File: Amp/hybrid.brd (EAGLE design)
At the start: 174 x 168.9 mm, 123 parts, among them IC1 TL071P, IC2 TL071P, IC3 LM317MABT-OUT, IC4 LM317MABT-OUT, J1 RCJ-21XXMILL, J2 NRJ3HF-1, J3 703W-00/54, Q1 BC560KINKED, Q10 BC560KINKED, Q11 BC560KINKED, Q12 BC560KINKED, Q13 BC556KINKED, Q14 BC550KINKED, Q15 BC550KINKED, Q16 BC560KINKED, Q17 BD140, Q18 BD139, Q19 KSP43, Q2 BC560KINKED, Q3 BC560KINKED, Q4 BC556KINKED, Q5 BC550KINKED, Q6 BC550KINKED, Q7 BC560KINKED, Q8 BD140, Q9 BD139, T1 TR-LP30-1600

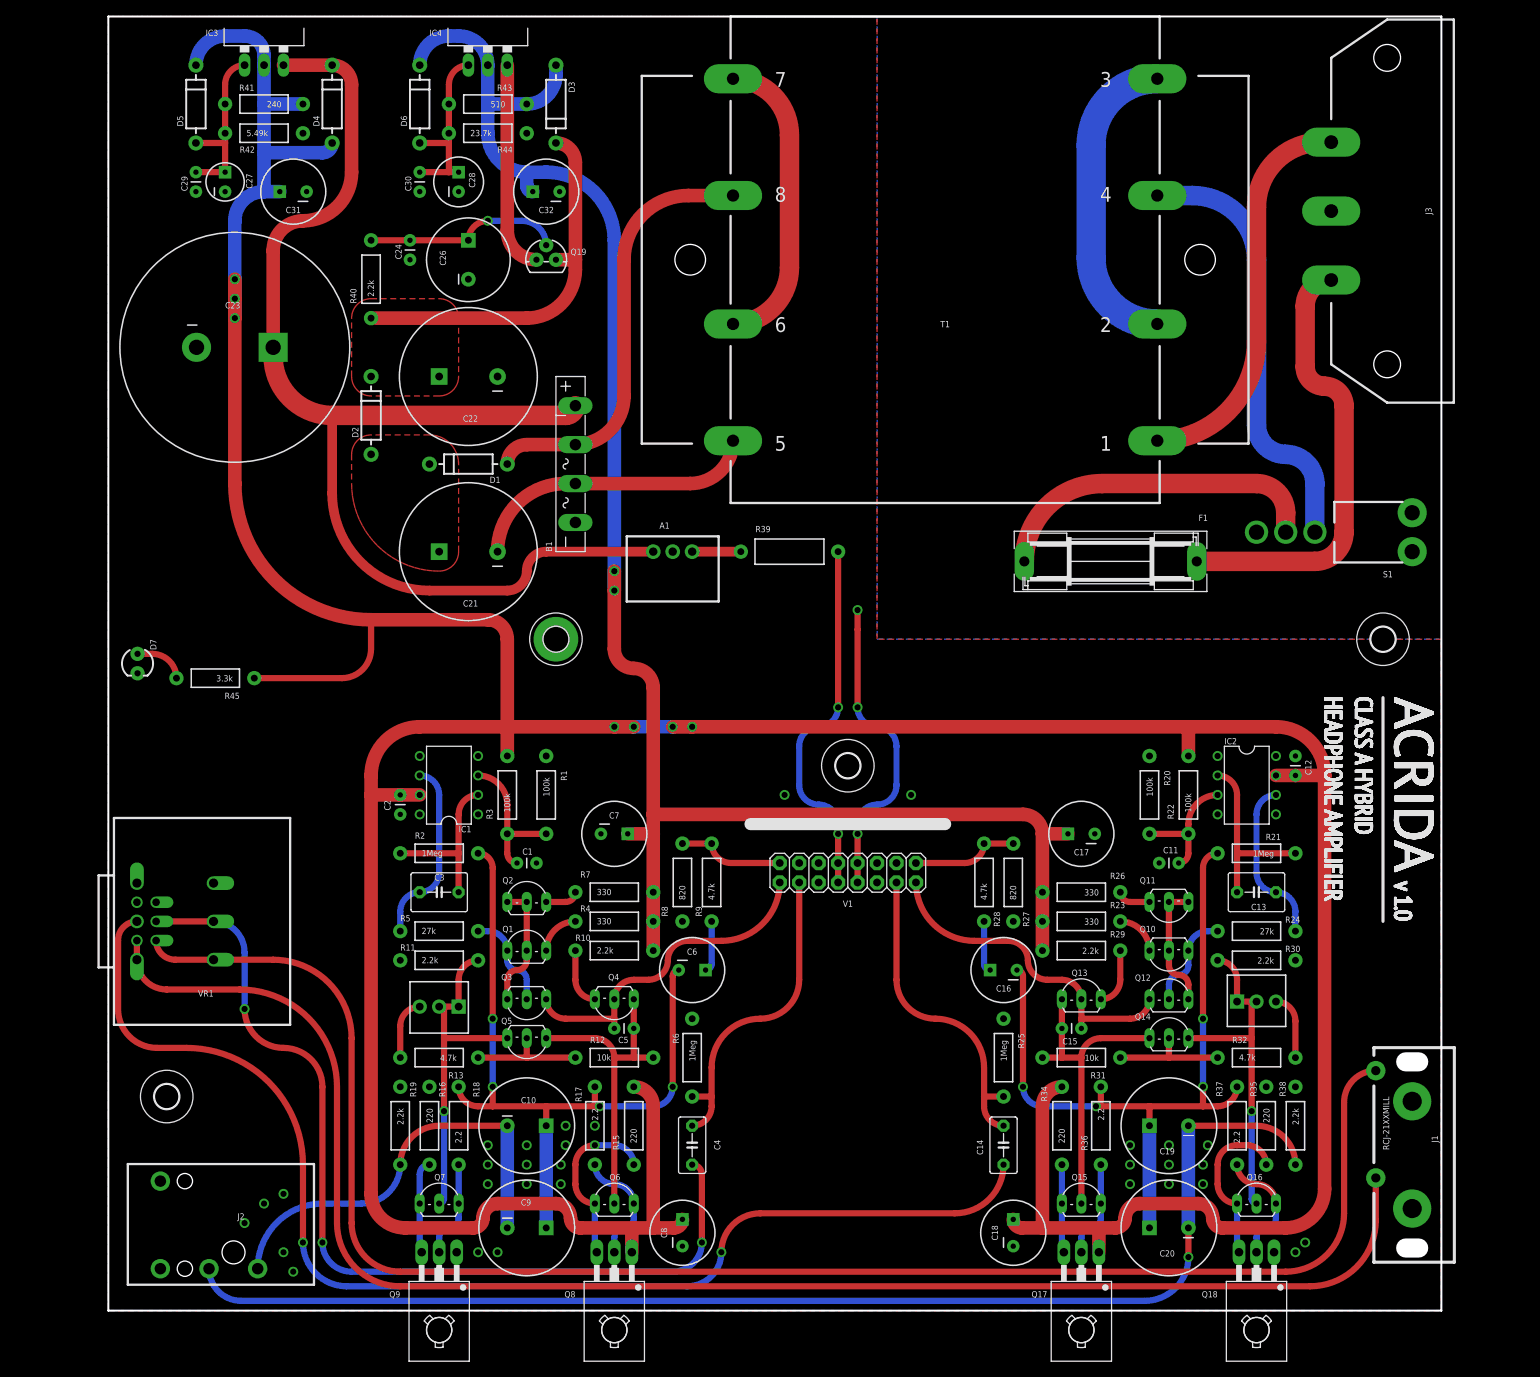
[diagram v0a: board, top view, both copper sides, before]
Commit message: Small changes
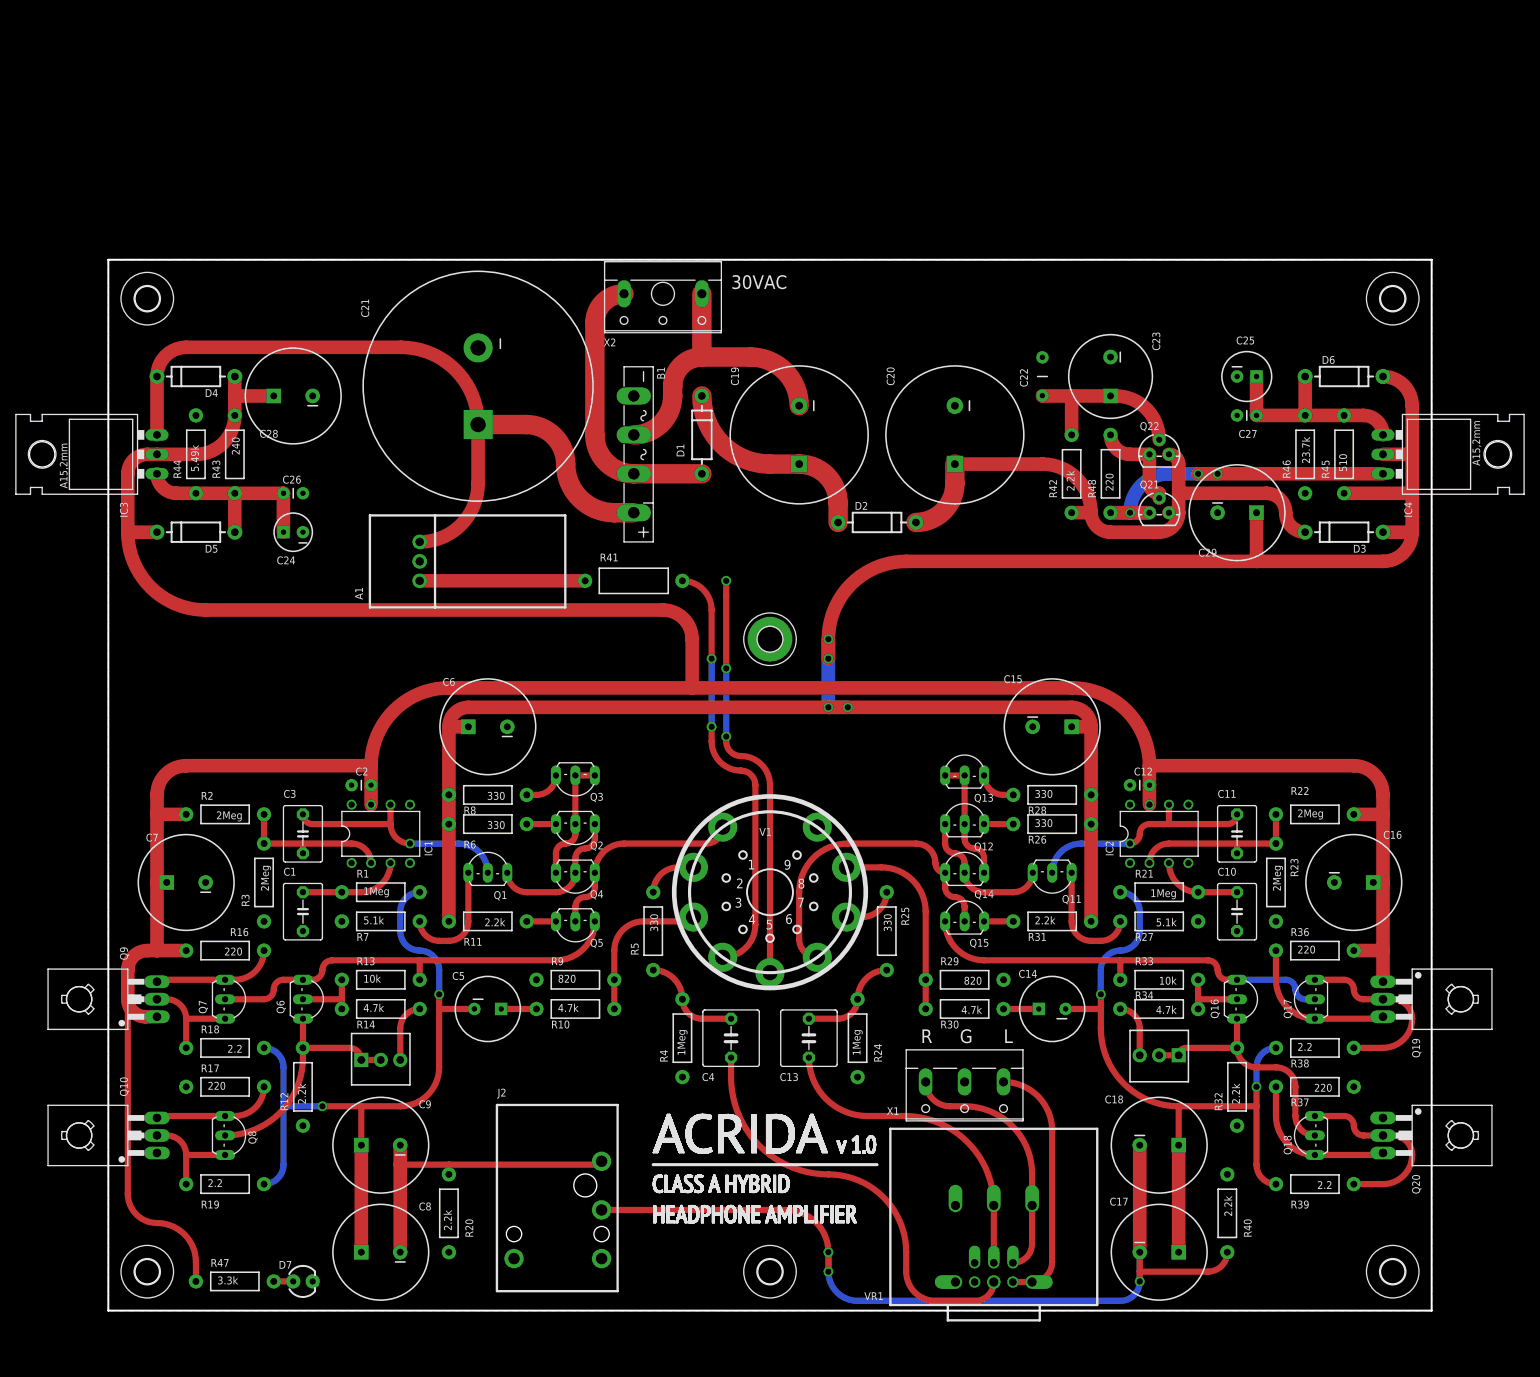
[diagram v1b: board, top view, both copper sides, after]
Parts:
- removed C30: 1uF, SparkFun-Capacitors:CAP-PTH-SMALL
- removed C31, C32: 47uF, my-cap:CPOL-RADIAL-8/3.5
- removed F1: (no value), fuse:SH22,5
- removed J1: RCJ-21XXMILL, my:RCJ-21-MILL
- removed J3: 703W-00/54, my-conn:703W-00/54
- removed S1: SW-M2012SA2W40, my-sw:SW-M2012S2A2G40
- removed T1: TR-LP30-1600, my-transformers:TR-LP30-1600
- removed U$1: ACRIDA-LOGO, my-logo:ACRIDA-LOGO
- removed U$2: (no value), my-logo:DANGER-LOGO
- added C25: 10uF, my-cap:CPOL-RADIAL-6.5/2.5
- added H1: MOUNT-PAD-ROUND3.2, holes:3,2-PAD
- added H6: MOUNT-HOLE3.2, holes:3,2
- added LOGO1: ACRIDA-LOGO, my-logo:ACRIDA-LOGO
- added Q20: BD139, transistor-npn:TO126
- added Q21, Q22: KSP43, my-tran:TO-92
- added R46: 23.7k, SparkFun-Resistors:AXIAL-0.4
- added R47: 3.3k, SparkFun-Resistors:AXIAL-0.4
- added R48: 220, SparkFun-Resistors:AXIAL-0.4
- added X1: (no value), con-wago-508:W237-3E
- added X2: (no value), con-wago-508:W237-2N
- C1, C11: value 0.1uF -> 1uF; device SparkFun-Capacitors:CAP-PTH-SMALL -> capacitor-wima:C5B5
- C10: value 470uF -> 1uF; device my-cap:CPOL-RADIAL-12.5/5 -> capacitor-wima:C5B5
- C12, C2: value 0.1uF -> 1uF
- C13: value 1uF -> 0.33u; device capacitor-wima:C5B5 -> capacitor-wima:C5B7.2
- C14: value 0.33u -> 100uF; device capacitor-wima:C5B3.5 -> my-cap:CPOL-RADIAL-8/3.5
- C15: value 10p -> 100uF; device SparkFun-Capacitors:CAP-PTH-SMALL -> my-cap:CPOL-RADIAL-12.5/5
- C16, C6: device my-cap:CPOL-RADIAL-8/3.5 -> my-cap:CPOL-RADIAL-12.5/5
- C17, C18, C8: value 47uF -> 470uF; device my-cap:CPOL-RADIAL-8/3.5 -> my-cap:CPOL-RADIAL-12.5/5
- C19, C20: device my-cap:CPOL-RADIAL-12.5/5 -> my-cap:CPOL-RADIAL-18/7.5
- C21: value 470uF -> 4700uF; device my-cap:CPOL-RADIAL-18/7.5 -> my-cap:CPOL-SNAPIN-30/10
- C22: value 470uF -> 1uF; device my-cap:CPOL-RADIAL-18/7.5 -> SparkFun-Capacitors:CAP-PTH-5MM
- C23: value 4700uF -> 47uF; device my-cap:CPOL-SNAPIN-30/10 -> my-cap:CPOL-RADIAL-12/5
- C24: value 1uF -> 10uF; device SparkFun-Capacitors:CAP-PTH-SMALL -> my-cap:CPOL-RADIAL-5/2.5
- C26: value 47uF -> 1uF; device my-cap:CPOL-RADIAL-12/5 -> SparkFun-Capacitors:CAP-PTH-SMALL
- C27: value 10uF -> 1uF; device my-cap:CPOL-RADIAL-5/2.5 -> SparkFun-Capacitors:CAP-PTH-SMALL
- C28: value 10uF -> 100uF; device my-cap:CPOL-RADIAL-6.5/2.5 -> my-cap:CPOL-RADIAL-12.5/5
- C29: value 1uF -> 100uF; device SparkFun-Capacitors:CAP-PTH-SMALL -> my-cap:CPOL-RADIAL-12.5/5
- C4: device capacitor-wima:C5B3.5 -> capacitor-wima:C5B7.2
- C5: value 10p -> 100uF; device SparkFun-Capacitors:CAP-PTH-SMALL -> my-cap:CPOL-RADIAL-8/3.5
- C7: value 47uF -> 100uF; device my-cap:CPOL-RADIAL-8/3.5 -> my-cap:CPOL-RADIAL-12.5/5
- H4: value MOUNT-PAD-ROUND3.2 -> MOUNT-HOLE3.2; device holes:3,2-PAD -> holes:3,2
- IC3, IC4: value LM317MABT-OUT -> LM317MABT; device my-reg:TO220L1-OUT -> my-reg:TO220L1
- Q1, Q11: value BC560KINKED -> KSP06KINKED
- Q10: value BC560KINKED -> BD139; device my-tran:TO92-BENT -> transistor-npn:TO126
- Q13, Q4: value BC556KINKED -> BC560KINKED
- Q14: value BC550KINKED -> BC560KINKED
- Q15, Q5: value BC550KINKED -> BC556KINKED
- Q16, Q7: value BC560KINKED -> BC550KINKED
- Q17: value BD140 -> BC550KINKED; device transistor-pnp:TO126 -> my-tran:TO92-BENT
- Q18: value BD139 -> BC560KINKED; device transistor-npn:TO126 -> my-tran:TO92-BENT
- Q19: value KSP43 -> BD140; device my-tran:TO-92 -> transistor-pnp:TO126
- Q8: value BD140 -> BC560KINKED; device transistor-pnp:TO126 -> my-tran:TO92-BENT
- Q9: value BD139 -> BD140; device transistor-npn:TO126 -> transistor-pnp:TO126
- R1: value 100k -> 1Meg
- R10, R30: value 2.2k -> 4.7k
- R12, R31: value 10k -> 2.2k
- R13: value 4.7k -> 10k
- R14: value 10k -> 4.7k; device SparkFun-Electromechanical:3362U-2 -> SparkFun-Resistors:AXIAL-0.4
- R15, R35: value 220 -> 10k; device SparkFun-Resistors:AXIAL-0.4 -> SparkFun-Electromechanical:3362U-2
- R17, R36, R37: value 2.2 -> 220
- R19, R38: value 2.2k -> 2.2
- R2: value 1Meg -> 2Meg
- R20: value 100k -> 2.2k
- R22, R3: value 100k -> 2Meg
- R23: value 330 -> 2Meg
- R24: value 27k -> 1Meg
- R25, R6: value 1Meg -> 330
- R27: value 820 -> 5.1k
- R28: value 4.7k -> 330
- R29: value 2.2k -> 820
- R32: value 4.7k -> 2.2k
- R33: device SparkFun-Electromechanical:3362U-2 -> SparkFun-Resistors:AXIAL-0.4
- R34: value 220 -> 4.7k
- R39: value 0.51 -> 2.2; device my-res:AXIAL-0.5 -> SparkFun-Resistors:AXIAL-0.4
- R4: value 330 -> 1Meg
- R41: value 240 -> 0.51; device SparkFun-Resistors:AXIAL-0.4 -> my-res:AXIAL-0.5
- R42: value 5.49k -> 2.2k
- R43: value 510 -> 240
- R44: value 23.7k -> 5.49k
- R45: value 3.3k -> 510
- R5: value 27k -> 330
- R7: value 330 -> 5.1k
- R8: value 820 -> 330
- R9: value 4.7k -> 820
- V1: device my-tubes:NOVAL-HORIZONTAL -> my-tubes:NOVAL-21MM
- moved R40 165.4 mm to (146.1, 12.7), turned to 270 degrees
- moved R45 150.2 mm to (161.3, 111.8), turned to 90 degrees
- moved Q19 149.6 mm to (171.4, 40.6), turned to 270 degrees
- moved C29 143.0 mm to (147.3, 104.1), turned to 0 degrees
- moved Q10 139.1 mm to (1.27, 22.9), turned to 90 degrees
- moved C27 138.0 mm to (149.9, 116.8), turned to 180 degrees
- moved IC4 132.4 mm to (170.2, 111.8), turned to 270 degrees
- moved VR1 127.9 mm to (115.6, -1.27), turned to 270 degrees
- moved D6 125.8 mm to (161.3, 121.9), turned to 0 degrees
- moved D3 117.1 mm to (161.3, 101.6), turned to 180 degrees
- moved H2 115.0 mm to (86.4, 5.08)
- moved R42 114.4 mm to (125.7, 109.2), turned to 90 degrees
- moved C23 114.4 mm to (130.8, 121.9), turned to 270 degrees
- moved R39 107.3 mm to (157.5, 16.5), turned to 180 degrees
- moved C20 107.2 mm to (110.5, 114.3), turned to 270 degrees
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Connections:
- removed net N$40: F1.1, J3.L
- removed net N$44: F1.2, S1.S
- removed net N$45: S1.UP-CONNECT, T1.4
- removed net P$1: J3.E
- new net N$47: Q1.1, R7.P$2
- new net N$48: Q11.1, R27.P$2
- net +6.3FIL: now also R41.P$2, V1.4; no longer R39.P$2, V1.7, V1.8
- net +LV: now also C21.1; no longer C23.1
- net AC_1: now also X2.2; no longer T1.8
- net AC_2: now also C19.2, X2.1; no longer C21.2, T1.5
- net CAT_L: now also R10.P$2, V1.3; no longer R8.P$2, V1.2
- net CAT_R: now also R29.P$2, R30.P$2, V1.8; no longer R27.P$2, R28.P$2, V1.16
- net FB_L: now also C5.2, C8.+, R1.P$2, R18.P$1, R19.P$2; no longer C10.+, C6.2, R17.P$1, R18.P$2, R2.P$2
- net FB_R: now also C14.2, C17.+, C18.+, R38.P$1, R39.P$2; no longer C16.2, C19.+, C20.+, R36.P$1, R37.P$2
- net FGND: now also V1.5; no longer V1.10, V1.9
- net GND: now also C10.1, C15.-, C16.-, C20.2, C21.2, C23.-, C25.2, C26.2, C28.-, C29.-, C6.-, C7.-, H1.B3,2, Q10.1, Q20.1, R12.P$1, R17.P$1, R23.P$2, R24.P$1, R29.P$1, R3.P$2, R32.P$1, R37.P$1, R4.P$1, R40.P$1, R46.P$2, R7.P$1, R9.P$1, X1.2; no longer C11.1, C17.2, C18.2, C23.2, C26.-, C28.2, C29.2, C30.2, C31.2, C32.2, C7.2, C8.2, H4.B3,2, J1.1, J1.3, Q18.1, Q9.1, R1.P$1, R11.P$1, R16.P$1, R19.P$1, R25.P$1, R30.P$1, R35.P$1, R38.P$1, R42.P$2, R6.P$1, R8.P$1, V1.11, V1.12, V1.14, V1.4, V1.5, V1.6
- net G_L: now also R4.P$2, R5.P$2; no longer R6.P$2, V1.3
- net G_R: now also C13.2, R24.P$2; no longer C14.2, V1.13
- net HT: now also C15.+, C29.+, C6.+, R11.P$2, R28.P$2, R31.P$2, R45.P$1, R6.P$2, R8.P$2; no longer C17.1, C32.1, C7.1, R10.P$2, R23.P$2, R29.P$2, R4.P$2, R43.P$1, R7.P$2
- net IN_L: now also VR1.1.2; no longer VR1.2.2.1, VR1.2.2.2
- net IN_L*: now also VR1.1.3.1, VR1.1.3.2, X1.1; no longer J1.4, VR1.2.3.1, VR1.2.3.2
- net IN_R: now also C13.1, VR1.2.2.1, VR1.2.2.2; no longer C14.1, VR1.1.2
- net IN_R*: now also VR1.2.3.1, VR1.2.3.2, X1.3; no longer J1.2, VR1.1.3.1, VR1.1.3.2
- net ISET_L: now also Q1.3, Q2.1, Q4.2; no longer Q1.1, Q3.2, R5.P$2
- net ISET_R: now also Q11.3, Q12.1, Q14.2; no longer Q10.1, Q12.2, R24.P$2
- net N$1: now also Q3.1, Q3.2, Q4.3; no longer Q1.2, Q2.1, Q3.3
- net N$10: now also R14.P$2, R15.3; no longer R13.P$2, R14.3
- net N$11: now also Q7.3, Q9.2, R18.P$2; no longer Q6.3, Q8.2, R17.P$2
- net N$12: now also Q6.3, Q8.2, R12.P$2, R15.1, R15.2; no longer Q5.3, Q7.2, R11.P$2, R14.1, R14.2
- net N$13: now also Q10.2, Q8.3, R19.P$1; no longer Q7.3, Q9.2, R18.P$1
- net N$14: now also Q7.1, Q9.3, R16.P$1; no longer Q6.1, Q8.3, R15.P$1
- net N$15: now also Q10.3, Q8.1, R17.P$2; no longer Q7.1, Q9.3, R16.P$2
- net N$16: now also Q13.3, R28.P$1; no longer Q11.3, R26.P$1
- net N$17: now also Q12.2, Q13.1, Q13.2, Q14.3; no longer Q10.2, Q11.1, Q11.2, Q12.3
- net N$18: now also Q21.2, Q22.1, R48.P$2; no longer J3.N, T1.1
- net N$19: now also C14.1, R30.P$1; no longer C16.1, R28.P$1
- net N$2: now also Q3.3, R8.P$1; no longer Q2.3, R7.P$1
- net N$20: now also Q15.3, R31.P$1; no longer Q13.3, R29.P$1
- net N$21: now also Q15.1, Q16.1, Q17.2, R33.P$2; no longer C15.2, Q13.1, Q14.1, Q15.2, R31.P$2
- net N$22: now also Q16.2, R33.P$1, R34.P$1; no longer Q14.2, R31.P$1, R32.P$1
- net N$23: now also R34.P$2, R35.3; no longer R32.P$2, R33.3
- net N$24: now also Q16.3, Q18.2, R32.P$2, R35.1, R35.2; no longer Q14.3, Q16.2, R30.P$2, R33.1, R33.2
- net N$25: now also Q17.3, Q19.2, R38.P$2; no longer Q15.3, Q17.2, R36.P$2
- net N$26: now also Q18.3, Q20.2, R39.P$1; no longer Q16.3, Q18.2, R37.P$1
- net N$27: now also Q17.1, Q19.3, R36.P$1; no longer Q15.1, Q17.3, R34.P$1
- net N$28: now also Q18.1, Q20.3, R37.P$2; no longer Q16.1, Q18.3, R35.P$2
- net N$29: now also Q1.2; no longer R5.P$1
- net N$3: now also Q2.3, R6.P$1; no longer Q1.3, R4.P$1
- net N$30: now also C24.1, C26.1, R43.P$2, R44.P$1; no longer C27.1, C29.1, R41.P$2, R42.P$1
- net N$31: now also C19.1; no longer C21.1
- net N$32: now also R41.P$1; no longer R39.P$1
- net N$33: now also C20.1, Q21.3, Q22.3, R42.P$1; no longer C22.1, Q19.3, R40.P$1
- net N$34: now also C22.1, C23.+, Q22.2, R42.P$2; no longer C24.1, C26.+, Q19.2, R40.P$2
- net N$35: now also R3.P$1
- net N$36: now also C25.1, C27.1, R45.P$2, R46.P$1; no longer C28.1, C30.1, R43.P$2, R44.P$1
- net N$37: now also Q21.1, R48.P$1; no longer Q19.1
- net N$38: now also R1.P$1; no longer R1.P$2, R3.P$1
- net N$39: now also Q12.3, R26.P$1; no longer Q10.3, R23.P$1
- net N$4: now also C5.1, R10.P$1; no longer C6.1, R9.P$1
- net N$41: now also C11.2, IC2.2, R22.P$1, R23.P$1; no longer C13.1, IC2.6, R24.P$1
- net N$42: now also C10.2, IC2.3; no longer C13.2, IC2.2
- net N$43: now also C11.1, IC2.6, Q11.2; no longer C11.2, IC2.3, R20.P$2, R22.P$1
- net N$46: now also R47.P$2; no longer R45.P$2
- net N$5: now also Q5.3, R11.P$1; no longer Q4.3, R10.P$1
- net N$6: now also R5.P$1, V1.2; no longer T1.2, T1.3
- net N$7: now also Q6.1, Q7.2, R13.P$2; no longer C5.2, Q4.1, Q6.2, R12.P$2
- net N$8: now also Q6.2, R14.P$1; no longer Q5.2, R12.P$1
- net N$9: now also R25.P$1, V1.7; no longer T1.6, T1.7
- net OUT_L: now also C8.-, R20.P$2; no longer C10.-, R19.P$2
- net OUT_R: now also C17.-, C18.-, R40.P$2; no longer C19.-, C20.-, R38.P$2
- net PL_L: now also Q4.1, Q5.2; no longer C5.1, Q3.1, Q4.2
- net PL_R: now also Q14.1, Q15.2, V1.6; no longer C15.1, Q12.1, Q13.2, V1.15
- net VCC: now also C16.+, C28.+, C7.+, Q19.1, Q9.1, R16.P$2, R2.P$2, R36.P$2, R43.P$1, R47.P$1; no longer C18.1, C31.1, C8.1, Q17.1, Q8.1, R15.P$2, R3.P$2, R34.P$2, R41.P$1, R45.P$1
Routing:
- net IN_L*: track 212.2 -> 32.3 mm
- net IN_R*: track 201.4 -> 31.5 mm
- net VCC: track 567.3 -> 422.7 mm, vias 7 -> 0
- net IN_R: track 155.5 -> 39.9 mm, vias 2 -> 0
- net IN_L: track 118.7 -> 51.4 mm, vias 3 -> 0
- net N$40: track 57.2 -> 0.00 mm
- net N$45: track 55.1 -> 0.00 mm
- net HT: track 228.9 -> 282.5 mm, vias 2 -> 4
- net +LV: track 152.3 -> 98.8 mm
- net OUT_R: track 165.2 -> 114.3 mm, vias 1 -> 3
- net N$44: track 42.4 -> 0.00 mm
- net N$18: track 49.1 -> 12.4 mm
- net N$6: track 39.2 -> 6.60 mm
- net N$9: track 38.1 -> 6.60 mm
- net G_R: track 40.1 -> 12.8 mm
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- removed copper zone on layer 1, net N$31
- removed copper zone on layer 1, net N$33
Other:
- board size 174 x 168.9 mm -> 172.7 x 137.2 mm
- board text added: "30VAC"
- board text added: "G"
- board text added: "L"
- board text added: "R"
